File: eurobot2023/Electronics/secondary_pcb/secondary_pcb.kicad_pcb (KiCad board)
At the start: 2 copper layers, 120.9 x 93.2 mm, 34 parts, among them IC1 CD74HCT125M96, IC2 SN74LVC126ADR, J1 PI40HAT, J10 Conn_01x02_Male, J11 MagneticEncoder, J12 Conn_01x07_Male, J13 MagneticEncoder, J14 Conn_01x03_Male, J15 Conn_01x02_Male, J2 Conn_01x02_Male, J3 Conn_01x02_Male, J4 Conn_01x02_Male, J5 Conn_01x02_Male, J6 Conn_01x02_Male, J7 Conn_01x02_Male, J9 22-03-5035, P1 R-78Bxx-2.0, P2 Amazon 5A stepdown, U1 MCP2515-xSO, U2 TJA1049T, U3 PCA9306D, U4 Pololu_MAX14870, U5 PCA9685PW

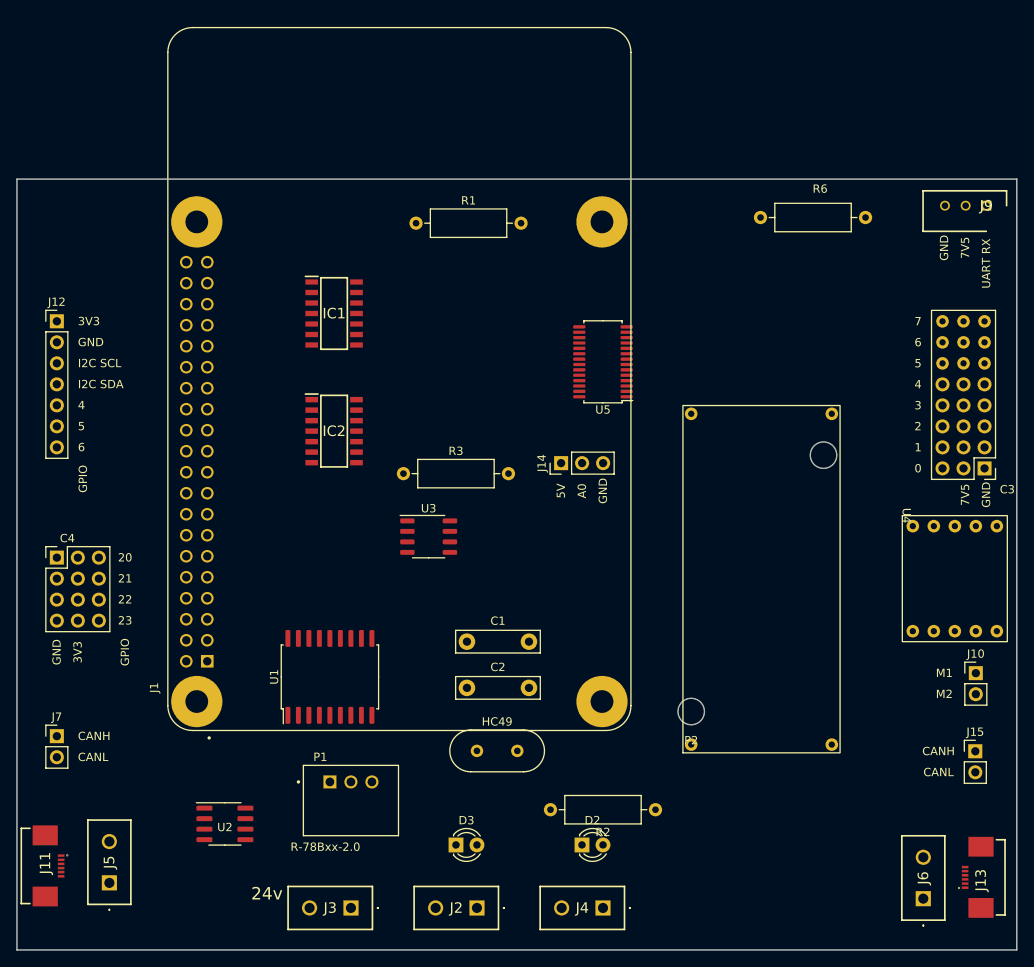
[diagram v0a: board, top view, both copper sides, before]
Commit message: Modify secondary pcb
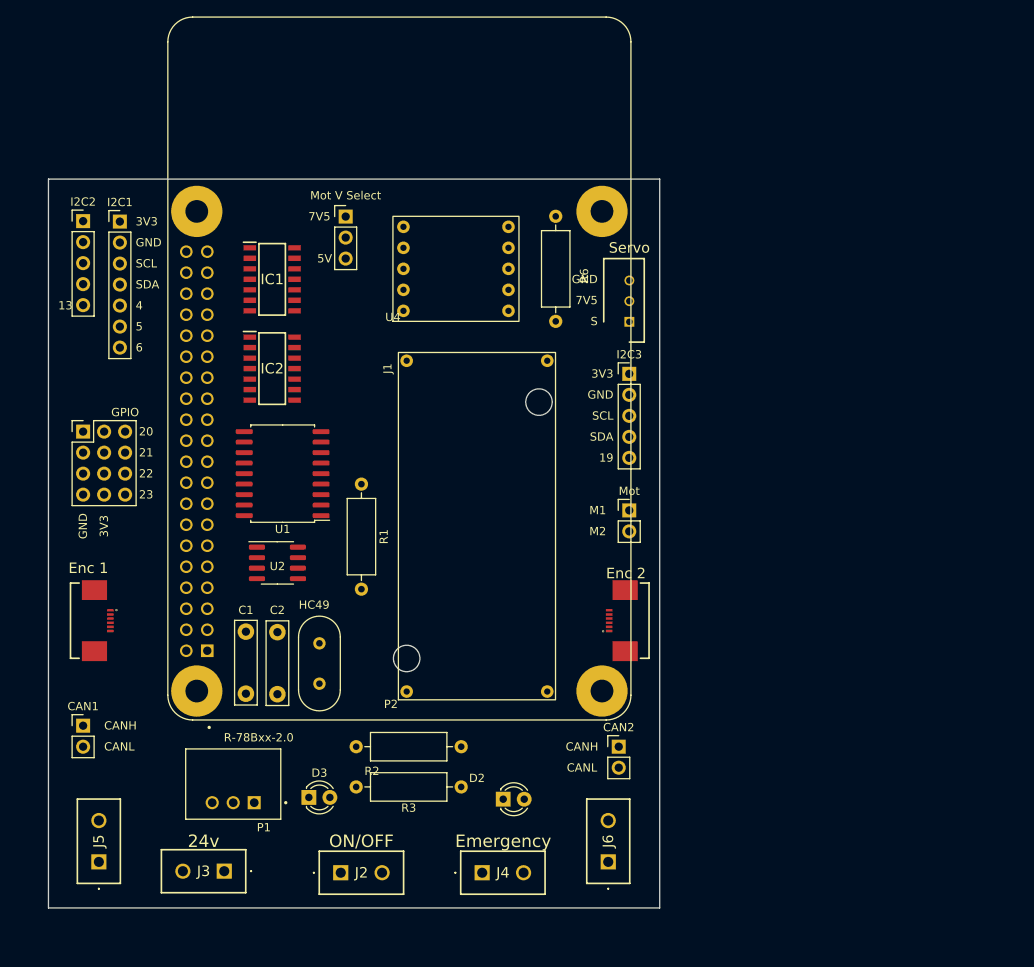
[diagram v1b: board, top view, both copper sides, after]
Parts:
- removed C3: Conn_03x08, MiAM:Pin_Header_Straight_3x08_Pitch2.54mm
- removed J14: Conn_01x03_Male, Connector_PinHeader_2.54mm:PinHeader_1x03_P2.54mm_Vertical
- removed U3: PCA9306D, Package_SO:SO-8_3.9x4.9mm_P1.27mm
- removed U5: PCA9685PW, Package_SO:TSSOP-28_4.4x9.7mm_P0.65mm
- added I2C2: Conn_01x05_Male, Connector_PinHeader_2.54mm:PinHeader_1x05_P2.54mm_Vertical, F.Cu at (71.8, 60.9)
- added I2C3: Conn_01x05_Male, Connector_PinHeader_2.54mm:PinHeader_1x05_P2.54mm_Vertical, F.Cu at (137.8, 79.4)
- added Mot V Select: Conn_01x03_Male, Connector_PinHeader_2.54mm:PinHeader_1x03_P2.54mm_Vertical, F.Cu at (103.5, 60.4)
- Enc 1: renamed from J11
- Enc 2: renamed from J13
- moved U4 65.9 mm to (109.2, 73.0), turned to 0 degrees
- moved Enc 2 53.1 mm to (135.9, 109.2)
- moved Mot 46.3 mm to (137.8, 95.9)
- moved Servo 45.4 mm to (137.8, 73.1), turned to -90 degrees
- moved CAN2 43.1 mm to (136.5, 124.5)
- moved J6 38.4 mm to (135.3, 138.4)
- moved R3 38.3 mm to (104.8, 129.3)
- moved P2 35.0 mm to (110.9, 117.8)
- moved R1 32.2 mm to (105.4, 92.7), turned to -90 degrees
- moved U2 32.2 mm to (95.2, 102.2)
- moved Enc 1 30.3 mm to (74.5, 109.2)
- moved C1 27.5 mm to (91.4, 118.0), turned to 90 degrees
- moved U1 25.2 mm to (95.9, 91.4), turned to 180 degrees
- moved R6 24.8 mm to (128.9, 60.3), turned to -90 degrees
- moved R2 24.7 mm to (117.5, 124.5)
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- renumbered J7 to CAN1, J15 to CAN2, C4 to GPIO, J12 to I2C1, J10 to Mot, J9 to Servo
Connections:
- J1 pad 33: unconnected-(J1-Pad33) -> /GPIO 13
- J1 pad 35: unconnected-(J1-Pad35) -> /GPIO 19
- U4 pad 9: +7.5V -> Net-(U4-Pad9)
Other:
- board size 120.9 x 93.2 mm -> 73.9 x 88.1 mm
- board text added: "13"
- board text added: "19"
- board text added: "Emergency"
- board text added: "ON/OFF"
- board text added: "S"
- board text added: "SCL"
- board text added: "SDA"
- board text removed: "0"
- board text removed: "1"
- board text removed: "2"
- board text removed: "3"
- board text removed: "7"
- board text removed: "A0"
- board text removed: "GPIO"
- board text removed: "I2C SCL"
- board text removed: "I2C SDA"
- board text removed: "UART RX"
